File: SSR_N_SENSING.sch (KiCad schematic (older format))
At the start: 17 parts, among them P8 CONN_01X02, Q1 BC850, U10 ACS722, U3 SHARPS202S02

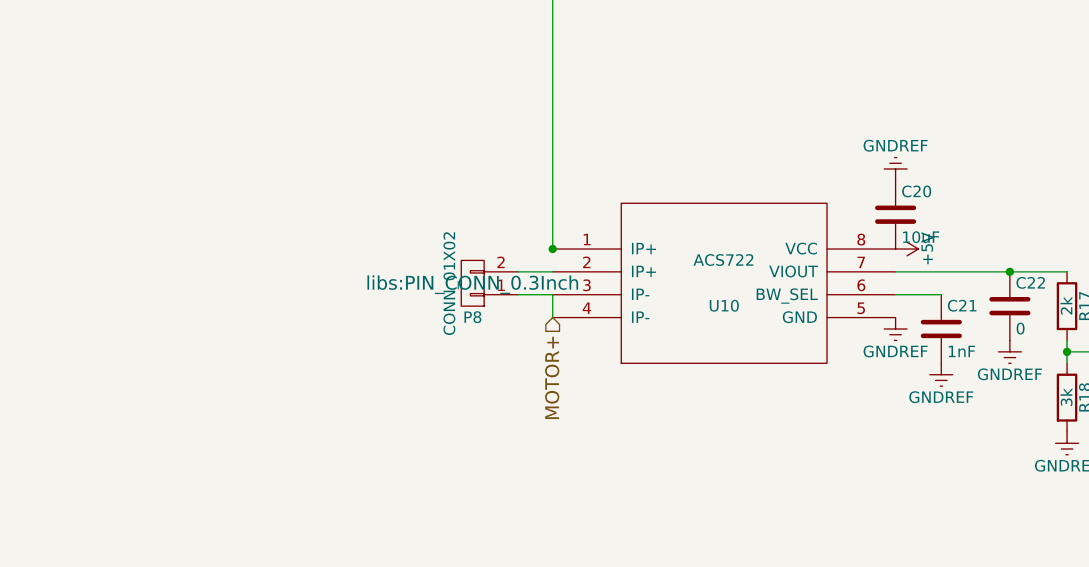
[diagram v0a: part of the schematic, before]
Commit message: small changes
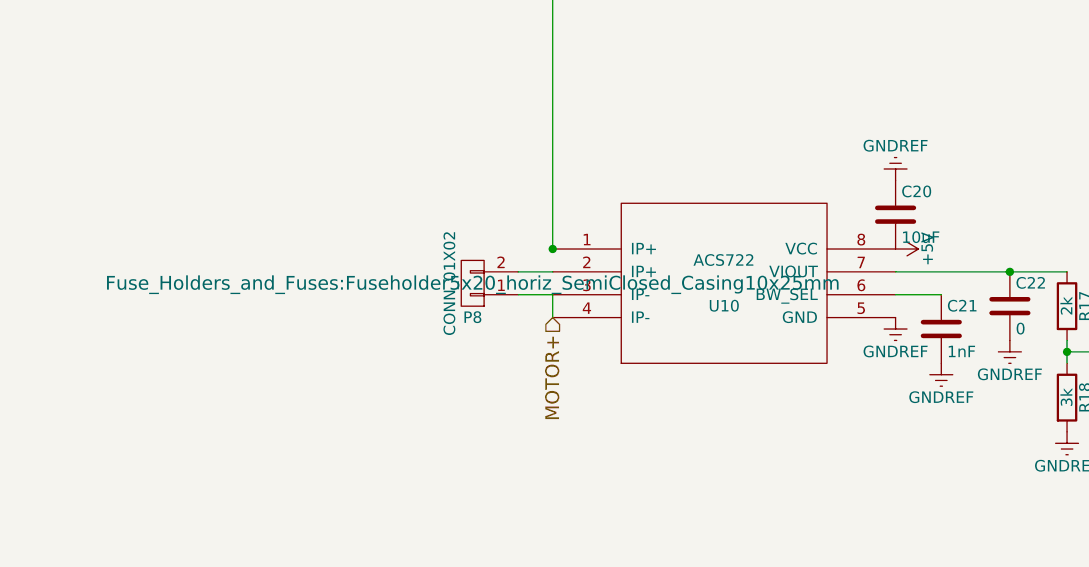
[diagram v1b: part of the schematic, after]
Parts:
- P8: footprint libs:PIN_CONN_0.3Inch -> Fuse_Holders_and_Fuses:Fuseholder5x20_horiz_SemiClosed_Casing10x25mm
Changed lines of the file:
@@
 LIBS:valves
 LIBS:analog_devices
-LIBS:libs
 LIBS:viztisztito-cache
 EELAYER 25 0
@@
 F 0 "P8" H 3100 4550 50  0000 C CNN
 F 1 "CONN_01X02" V 3200 4400 50  0000 C CNN
-F 2 "libs:PIN_CONN_0.3Inch" H 3100 4400 60  0000 C CNN
+F 2 "Fuse_Holders_and_Fuses:Fuseholder5x20_horiz_SemiClosed_Casing10x25mm" H 3100 4400 60  0000 C CNN
 F 3 "" H 3100 4400 60  0000 C CNN
 	1    3100 4400
